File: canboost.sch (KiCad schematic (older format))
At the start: 19 parts, among them IC1 MCP2551-I/SN, P1 CONN_10X2, P2 CONN_10X2, P3 CONN_2

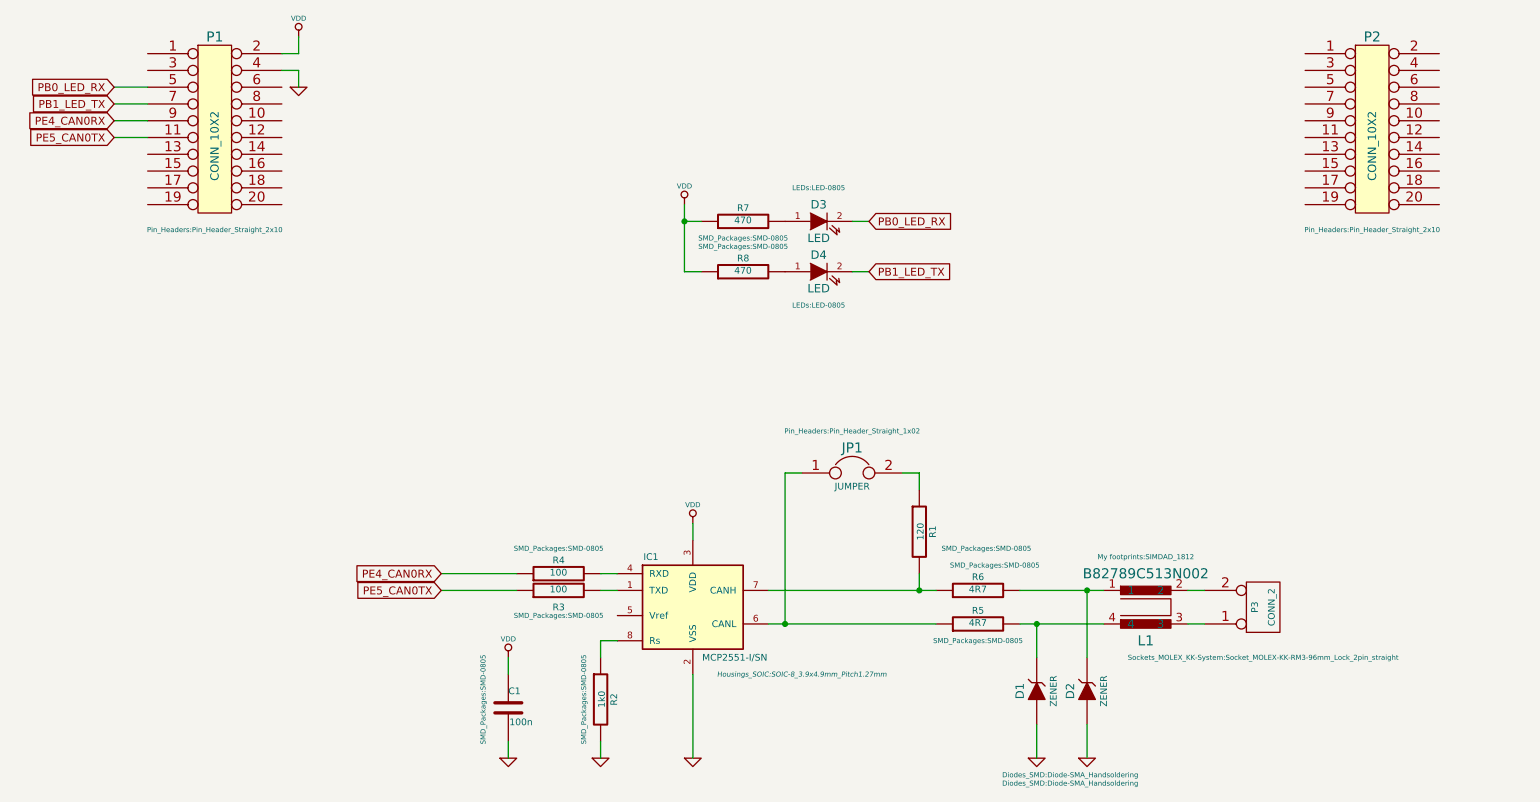
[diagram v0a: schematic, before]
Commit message: layout complete (v0.10)
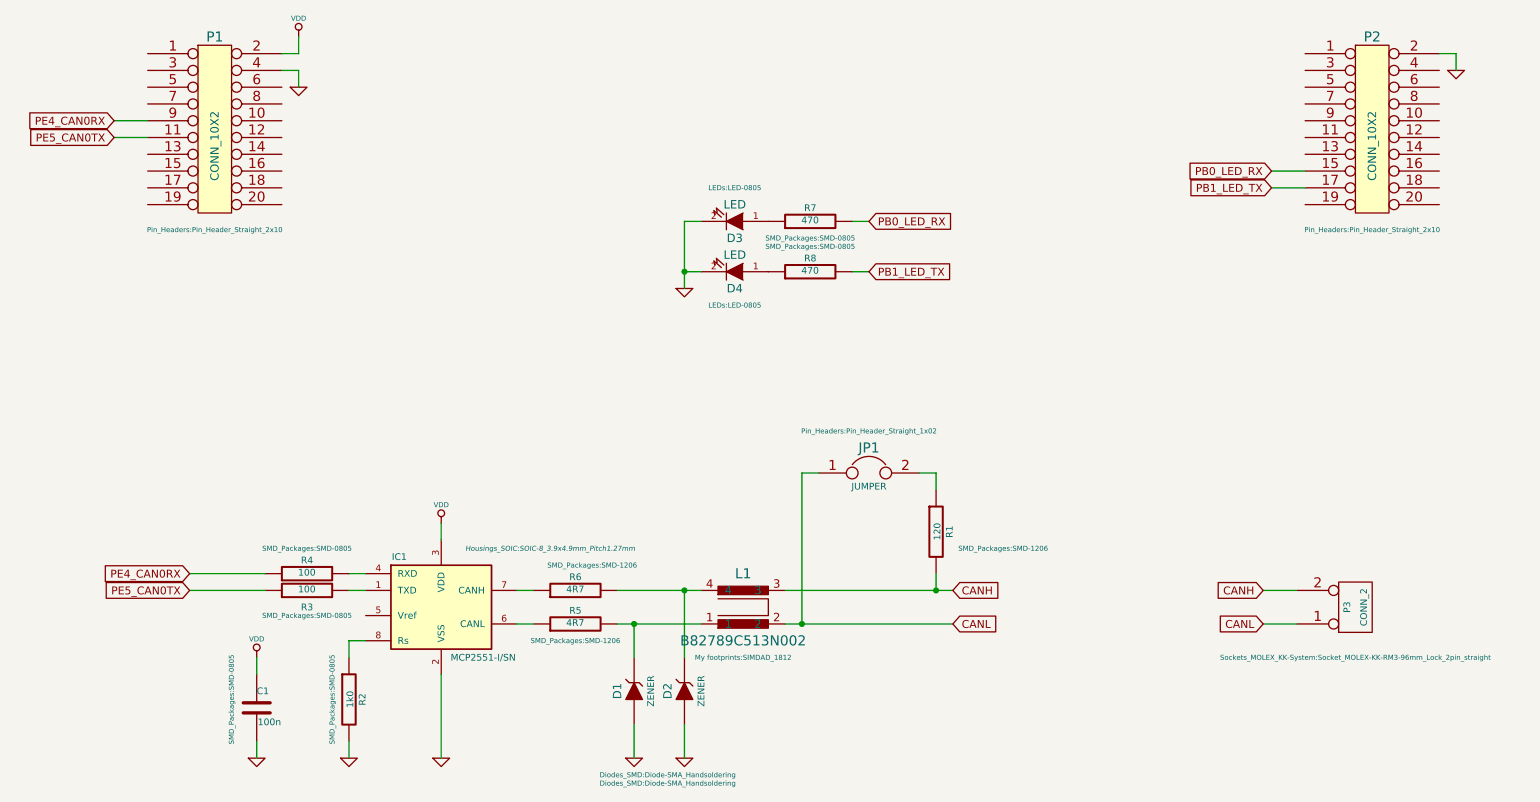
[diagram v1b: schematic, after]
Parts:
- R1, R5, R6: footprint SMD_Packages:SMD-0805 -> SMD_Packages:SMD-1206
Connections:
- net GND: now also D3.2 (K), D4.2 (K), P2.2 (P2)
- net PB0_LED_RX: now also P2.15 (P15), R7.2; no longer D3.2 (K), P1.5 (P5)
- net PB1_LED_TX: now also P2.17 (P17), R8.2; no longer D4.2 (K), P1.7 (P7)
- net VDD: no longer R7.1, R8.1
- net at IC1.6 (CANL), R5.1: no longer JP1.1
- net at IC1.7 (CANH), R6.1: no longer R1.2
- net CANH: now reaches L1.3
- net CANH: now also P3.2 (PM), R1.2; no longer P3.1 (P1)
- net CANL: now reaches L1.2
- net CANL: now also JP1.1, P3.1 (P1); no longer P3.2 (PM)
- net at D2.2 (K), R6.2: now also L1.4; no longer L1.1
- net at D1.2 (K), R5.2: now also L1.1; no longer L1.4
- net at D3.1 (A): now also R7.1; no longer R7.2
- net at D4.1 (A): now also R8.1; no longer R8.2
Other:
- moved on the sheet: C1, D1, D2, D3, D4, IC1, JP1, L1, P3, R1, R2, R3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
